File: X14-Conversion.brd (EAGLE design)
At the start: 50.8 x 62.9 mm, 22 parts, among them U1 BUCK,LM2678S-ADJ

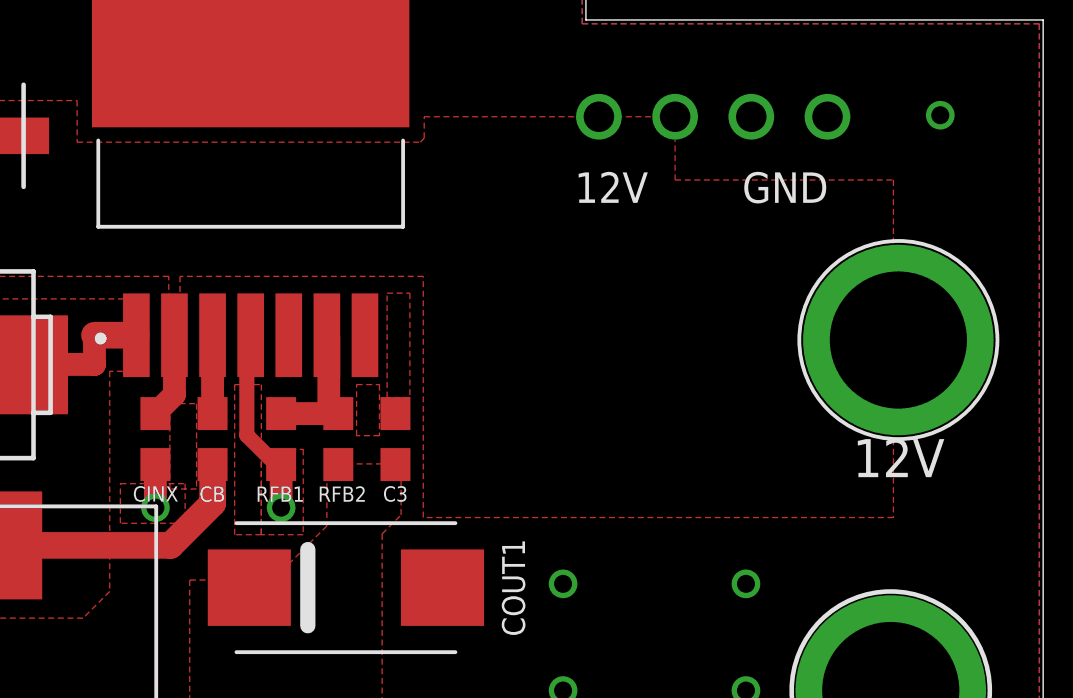
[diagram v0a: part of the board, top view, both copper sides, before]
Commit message: Update X14-Conversion.brd
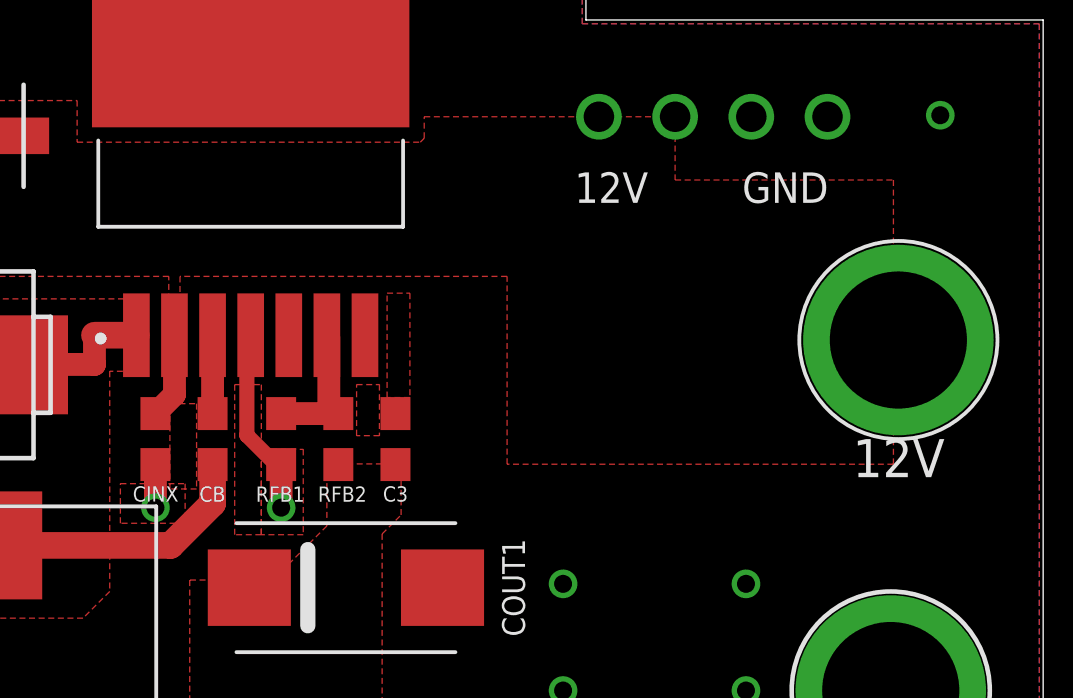
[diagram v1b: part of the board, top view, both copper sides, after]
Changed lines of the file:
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@@
 <wire x1="24.257" y1="42.705" x2="24.257" y2="39.497" width="0.508" layer="1"/>
 <wire x1="24.257" y1="39.497" x2="25.4" y2="38.354" width="0.508" layer="1"/>
-<wire x1="25.4" y1="38.52" x2="29.21" y2="40.22" width="0" layer="19" extent="1-1"/>
 </signal>
 <signal name="3.3V">
@@
 <vertex x="38.5318" y="48.006"/>
 <vertex x="45.8089" y="48.006"/>
-<vertex x="45.8089" y="36.7538"/>
-<vertex x="30.1371" y="36.7538"/>
-<vertex x="30.1371" y="44.7929"/>
+<vertex x="45.8089" y="38.5318"/>
+<vertex x="32.9311" y="38.5318"/>
+<vertex x="32.9311" y="44.7929"/>
 <vertex x="22.02815" y="44.7929"/>
 <vertex x="22.02815" y="41.783"/>
